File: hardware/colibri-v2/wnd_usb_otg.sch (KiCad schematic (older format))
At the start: 17 parts

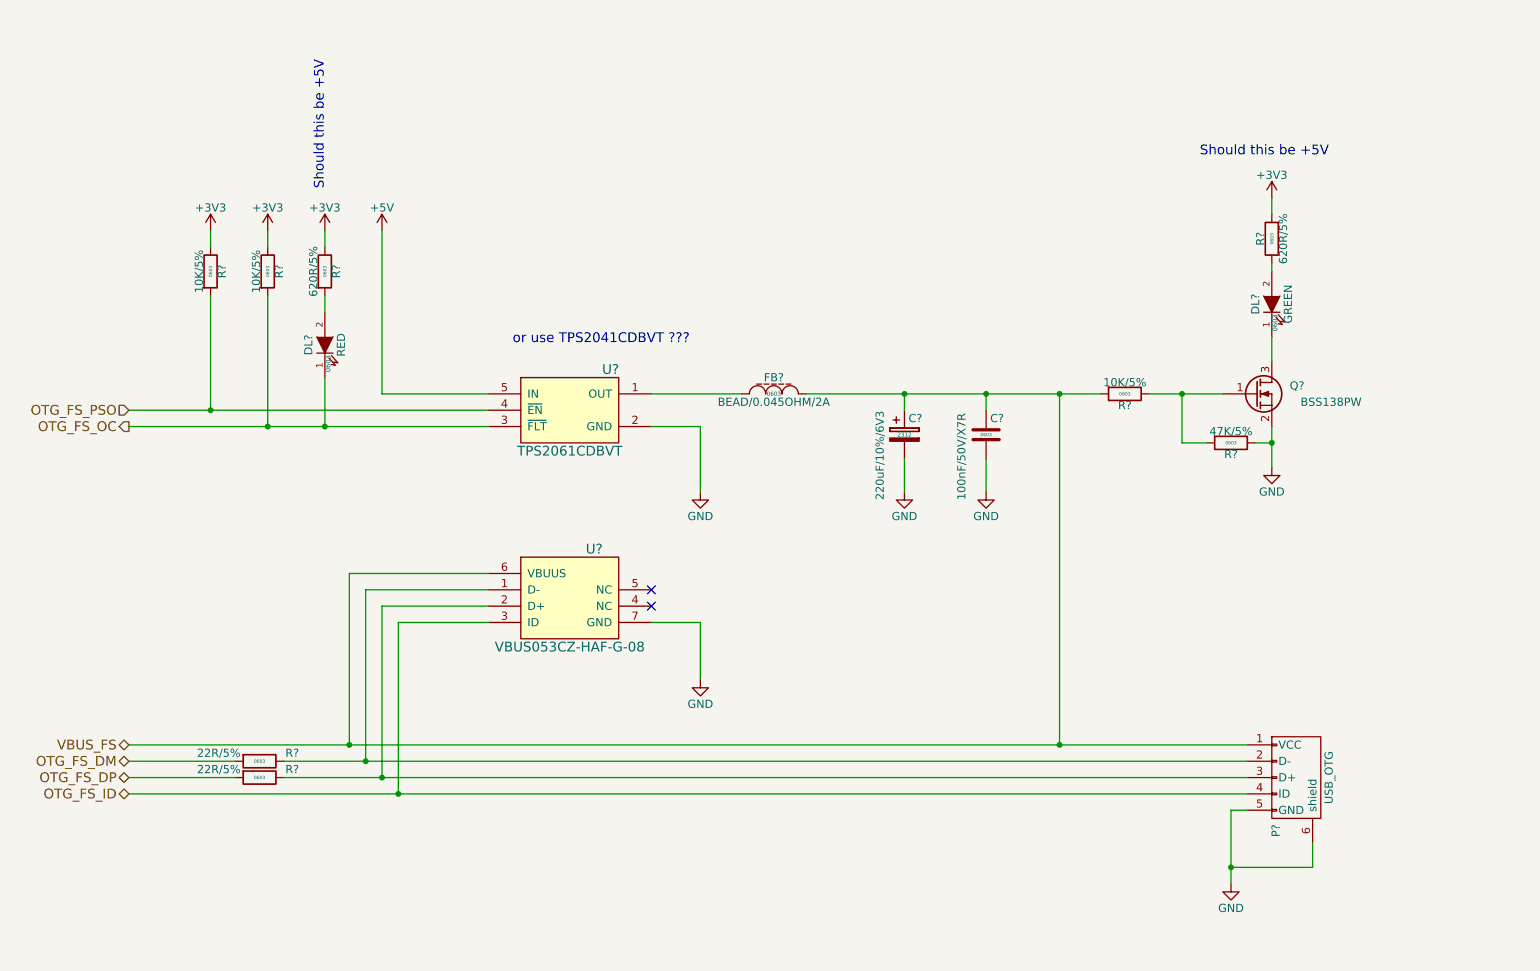
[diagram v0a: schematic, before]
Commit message: Work on PWM, USB, MEMS, Power
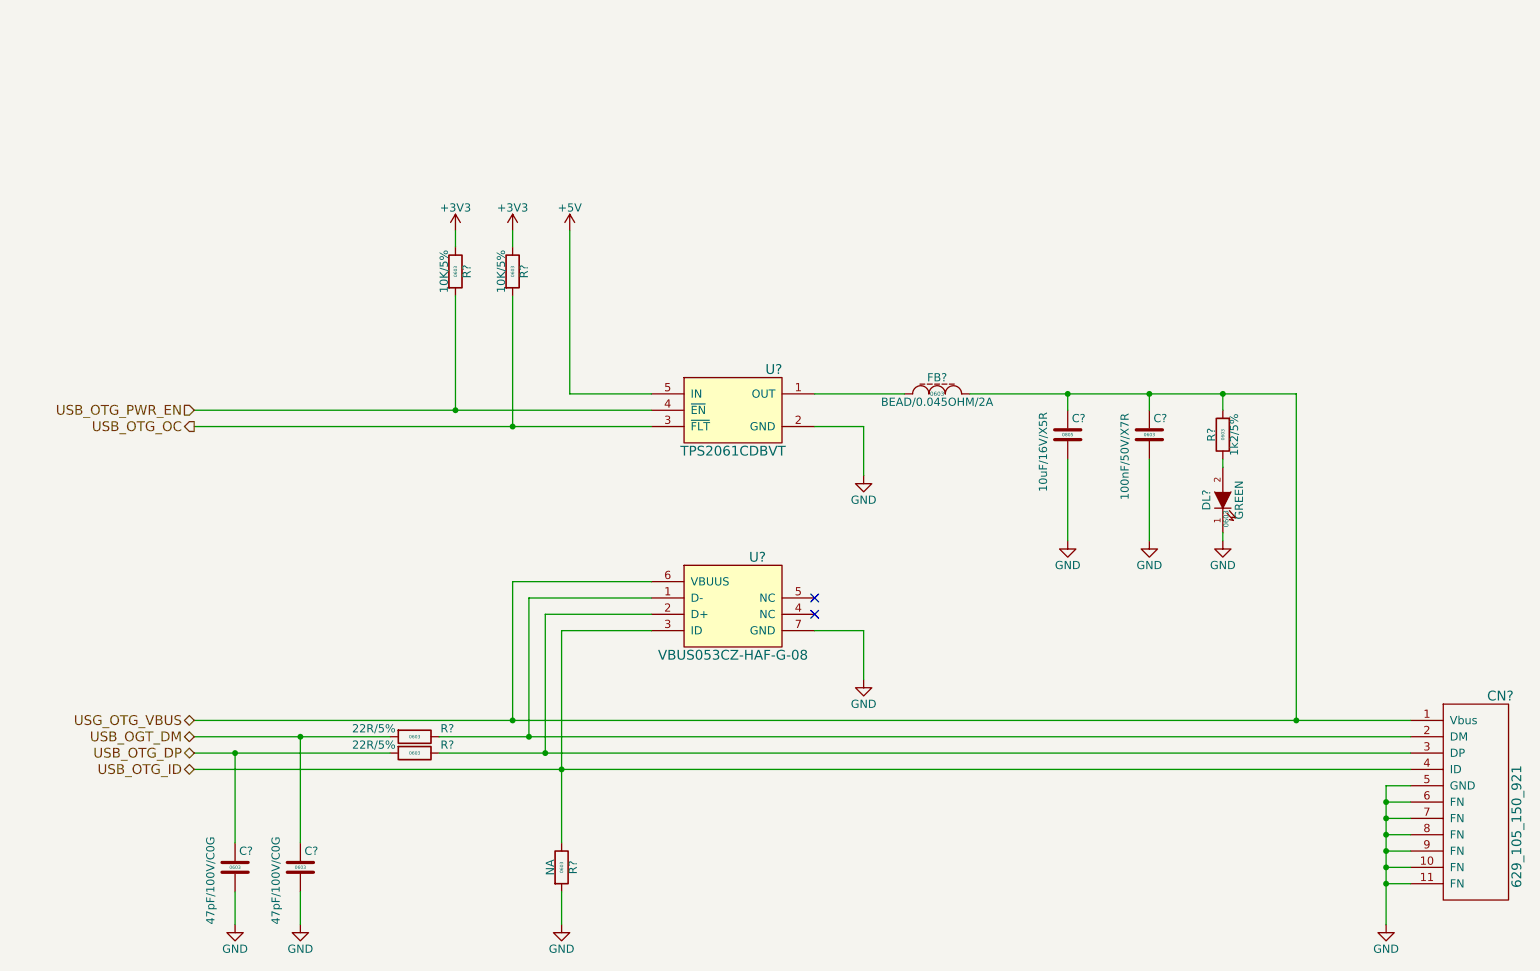
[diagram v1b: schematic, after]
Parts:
- removed C?: 100nF/50V/X7R, Capacitors_SMD:C_0603, symbol C_SMT
- removed C?: 220uF/10%/6V3, Capacitors_Tantalum_SMD:TantalC_SizeC_EIA-6032_Reflow, symbol CP_SMT
- removed DL?: GREEN, LEDs:LED-0603, symbol LED_SMT
- removed DL?: RED, LEDs:LED-0603, symbol LED_SMT
- removed FB?: BEAD/0.045OHM/2A, Resistors_SMD:R_0603, symbol FB_SMT
- removed P?: USB_OTG, symbol USB_OTG
- removed Q?: BSS138PW, symbol Q_NMOS_GSD
- removed R? (x3): 10K/5%, Resistors_SMD:R_0603, symbol R_SMT
- removed R? (x2): 620R/5%, Resistors_SMD:R_0603, symbol R_SMT
- removed R? (x2): 22R/5%, Resistors_SMD:R_0603, symbol R_SMT
- removed R?: 47K/5%, Resistors_SMD:R_0603, symbol R_SMT
- removed U?: VBUS053CZ-HAF-G-08, symbol VBUS053CZ-HAF-G-08
- removed U?: TPS2061CDBVT, symbol TPS2061CDBVT
- added C?: 10uF/16V/X5R, Capacitors_SMD:C_0603, symbol C_SMT
- added C?: 100nF/50V/X7R, Capacitors_SMD:C_0603, symbol C_SMT
- added C? (x2): 47pF/100V/C0G, Capacitors_SMD:C_0603, symbol C_SMT
- added CN?: 629_105_150_921, symbol 629_105_150_921
- added DL?: GREEN, LEDs:LED-0603, symbol LED_SMT
- added FB?: BEAD/0.045OHM/2A, Resistors_SMD:R_0603, symbol FB_SMT
- added R? (x2): 10K/5%, Resistors_SMD:R_0603, symbol R_SMT
- added R? (x2): 22R/5%, Resistors_SMD:R_0603, symbol R_SMT
- added R?: 1k2/5%, Resistors_SMD:R_0603, symbol R_SMT
- added R?: NA, Resistors_SMD:R_0603, symbol R_SMT
- added U?: VBUS053CZ-HAF-G-08, symbol VBUS053CZ-HAF-G-08
- added U?: TPS2061CDBVT, symbol TPS2061CDBVT
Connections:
- net +3V3: now also R?.1, R?.1
- net +5V: now also U?.5 (IN)
- net GND: now also C?.2, C?.2, C?.2, C?.2, CN?.10 (FN), CN?.11 (FN), CN?.5 (GND), CN?.6 (FN), CN?.7 (FN), CN?.8 (FN), CN?.9 (FN), DL?.1 (K), R?.2, U?.2 (GND), U?.7 (GND)
- new net: CN?.2 (DM), R?.1, U?.1 (D-)
- new net: CN?.3 (DP), R?.1, U?.2 (D+)
- new net: FB?.1, U?.1 (OUT)
- new net: DL?.2 (A), R?.1
- new net USB_OGT_DM: C?.1, R?.2
- new net USB_OTG_DP: C?.1, R?.2
- new net USB_OTG_ID: CN?.4 (ID), R?.1, U?.3 (ID)
- new net USB_OTG_OC: R?.2, U?.3 (~FLT)
- new net USB_OTG_PWR_EN: R?.2, U?.4 (~EN)
- new net USG_OTG_VBUS: C?.1, C?.1, CN?.1 (Vbus), FB?.2, R?.2, U?.6 (VBUUS)
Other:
- note removed: "Should this be +5V"
- note removed: "or use TPS2041CDBVT ???"
